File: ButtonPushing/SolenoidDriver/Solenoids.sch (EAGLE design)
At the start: 29 parts, among them U1 TLE94112EL

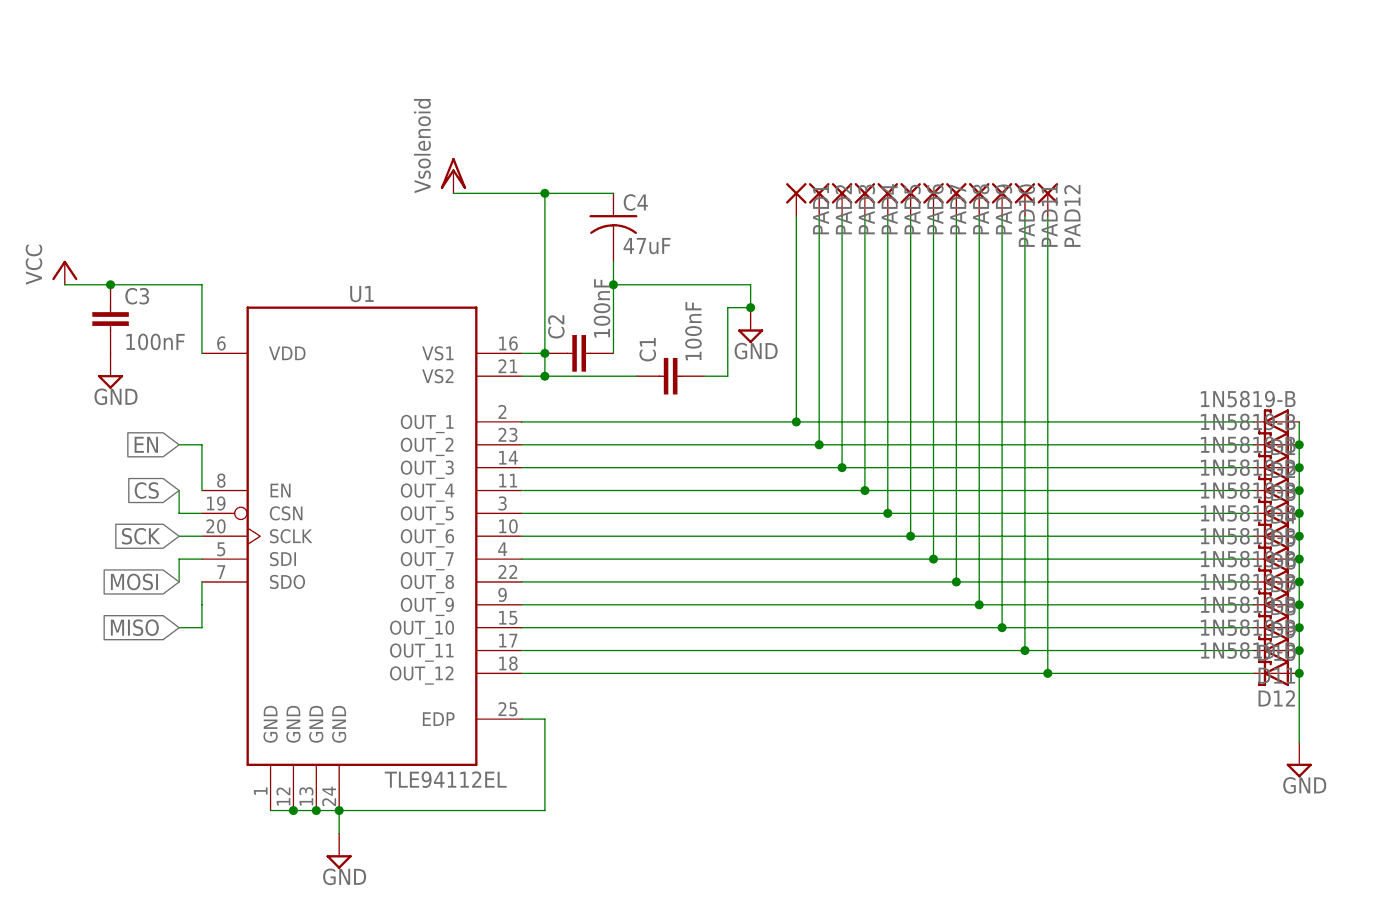
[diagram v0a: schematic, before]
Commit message: Fully routed PCB
Basically done, but needs to be checked over
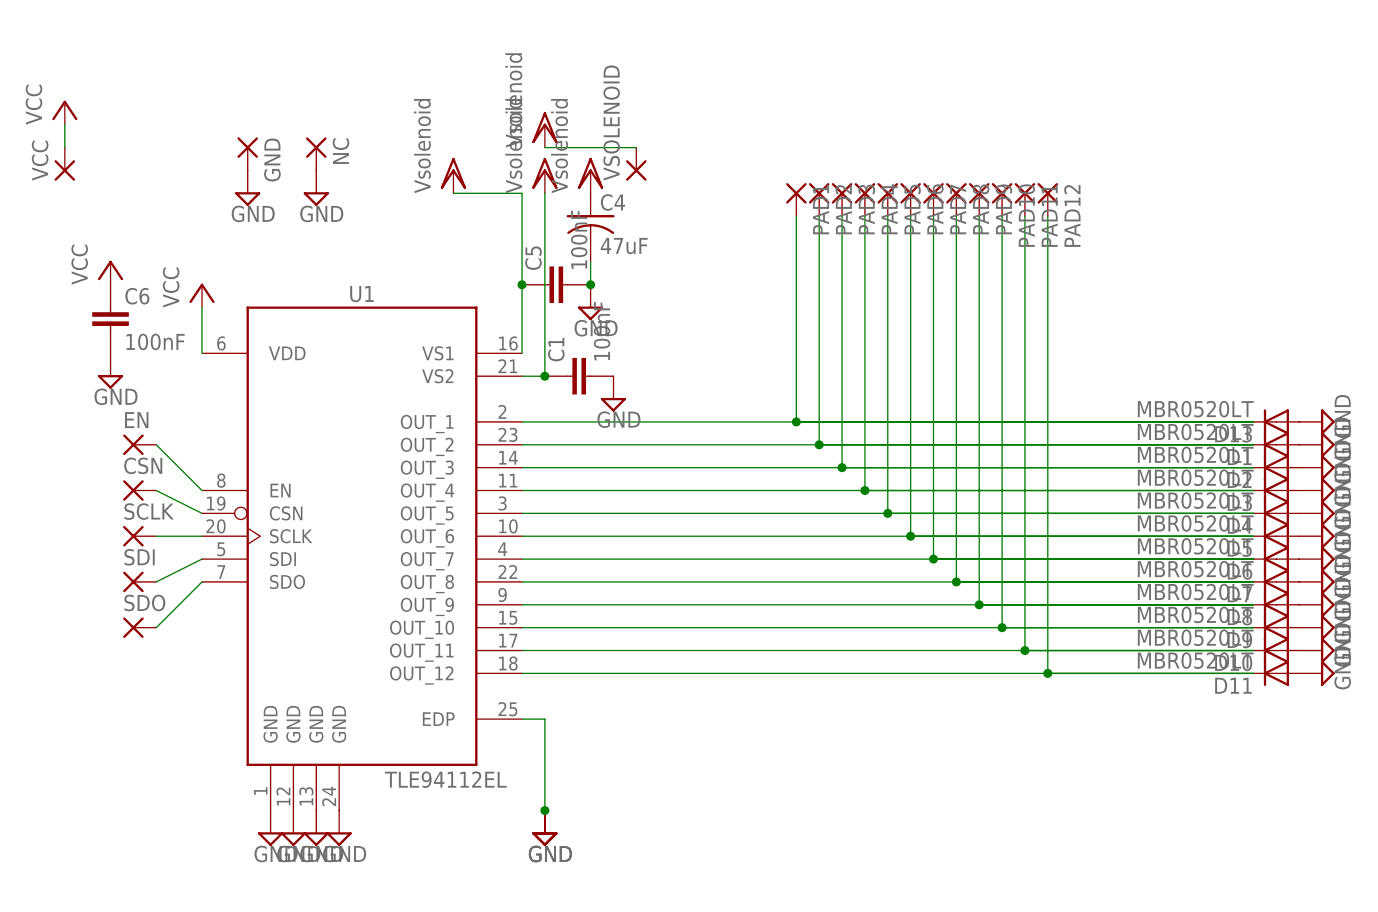
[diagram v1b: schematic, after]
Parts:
- removed C2, C3: 100nF, rcl:C-EUC0402
- removed D12: 1N5819-B, diode:1N5819-B
- added C5, C6: 100nF, rcl:C-EUC0402K
- added CSN, EN, GND, NC, SCLK, SDI, SDO, VCC, VSOLENOID: (no value), wirepad:1,6/0,8
- added D13: MBR0520LT, diode:MBR0520LT
- C1: device rcl:C-EUC0402 -> rcl:C-EUC0402K
- D1, D10, D11, D2, D3, D4, D5, D6, D7, D8, D9: value 1N5819-B -> MBR0520LT; device diode:1N5819-B -> diode:MBR0520LT
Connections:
- removed net CS: U1.CSN
- removed net EN: U1.EN
- removed net MISO: U1.SDO
- removed net MOSI: U1.SDI
- removed net SCK: U1.SCLK
- removed net SOLENOID: C1.1, C2.1, C4.1, U1.VS1, U1.VS2
- new net N$22: EN.P, U1.EN
- new net N$23: CSN.P, U1.CSN
- new net N$24: SCLK.P, U1.SCLK
- new net N$25: SDI.P, U1.SDI
- new net N$26: SDO.P, U1.SDO
- new net VDD: C1.1, C4.1, C5.1, U1.VS1, U1.VS2, VSOLENOID.P
- net GND: now also C5.2, C6.2, D13.A, GND.P, NC.P; no longer C2.2, C3.2, D12.A
- net N$1: now also D13.C; no longer D1.C
- net N$10: now also D9.C; no longer D10.C
- net N$11: now also D10.C; no longer D11.C
- net N$12: now also D11.C; no longer D12.C
- net N$2: now also D1.C; no longer D2.C
- net N$3: now also D2.C; no longer D3.C
- net N$4: now also D3.C; no longer D4.C
- net N$5: now also D4.C; no longer D5.C
- net N$6: now also D5.C; no longer D6.C
- net N$7: now also D6.C; no longer D7.C
- net N$8: now also D7.C; no longer D8.C
- net N$9: now also D8.C; no longer D9.C
- net VCC: now also C6.1, VCC.P; no longer C3.1
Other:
- moved on the sheet: C1, C4
